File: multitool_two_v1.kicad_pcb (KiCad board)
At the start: 2 copper layers, 144.8 x 119.4 mm, 69 parts, among them J1 Conn_02x08_Odd_Even, SW1 SW_Push, SW2 SW_Push, SW3 SW_Push, SW4 SW_Push, SW5 SW_Push, SW6 SW_Push, SW7 SW_Push, SW8 SW_Push, U1 4017, U2 74LS74, U3 74LS74, U4 74LS74, U5 74LS74, U6 74HCT00, U7 74HCT00, U8 74HCT00

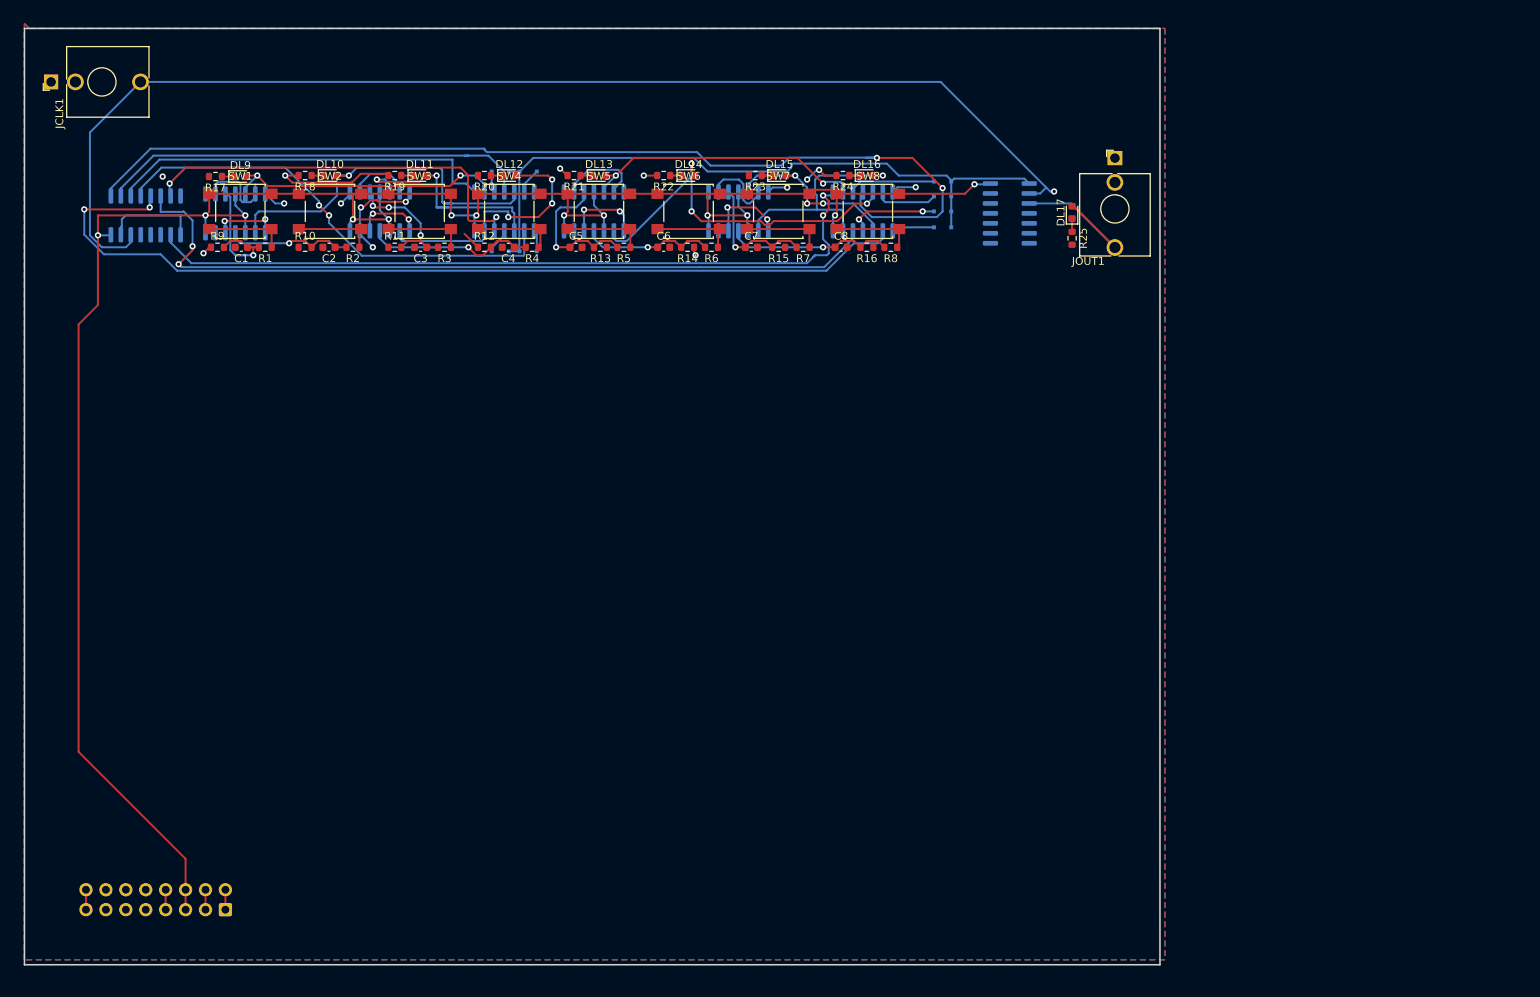
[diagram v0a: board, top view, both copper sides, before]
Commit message: committing with a bug
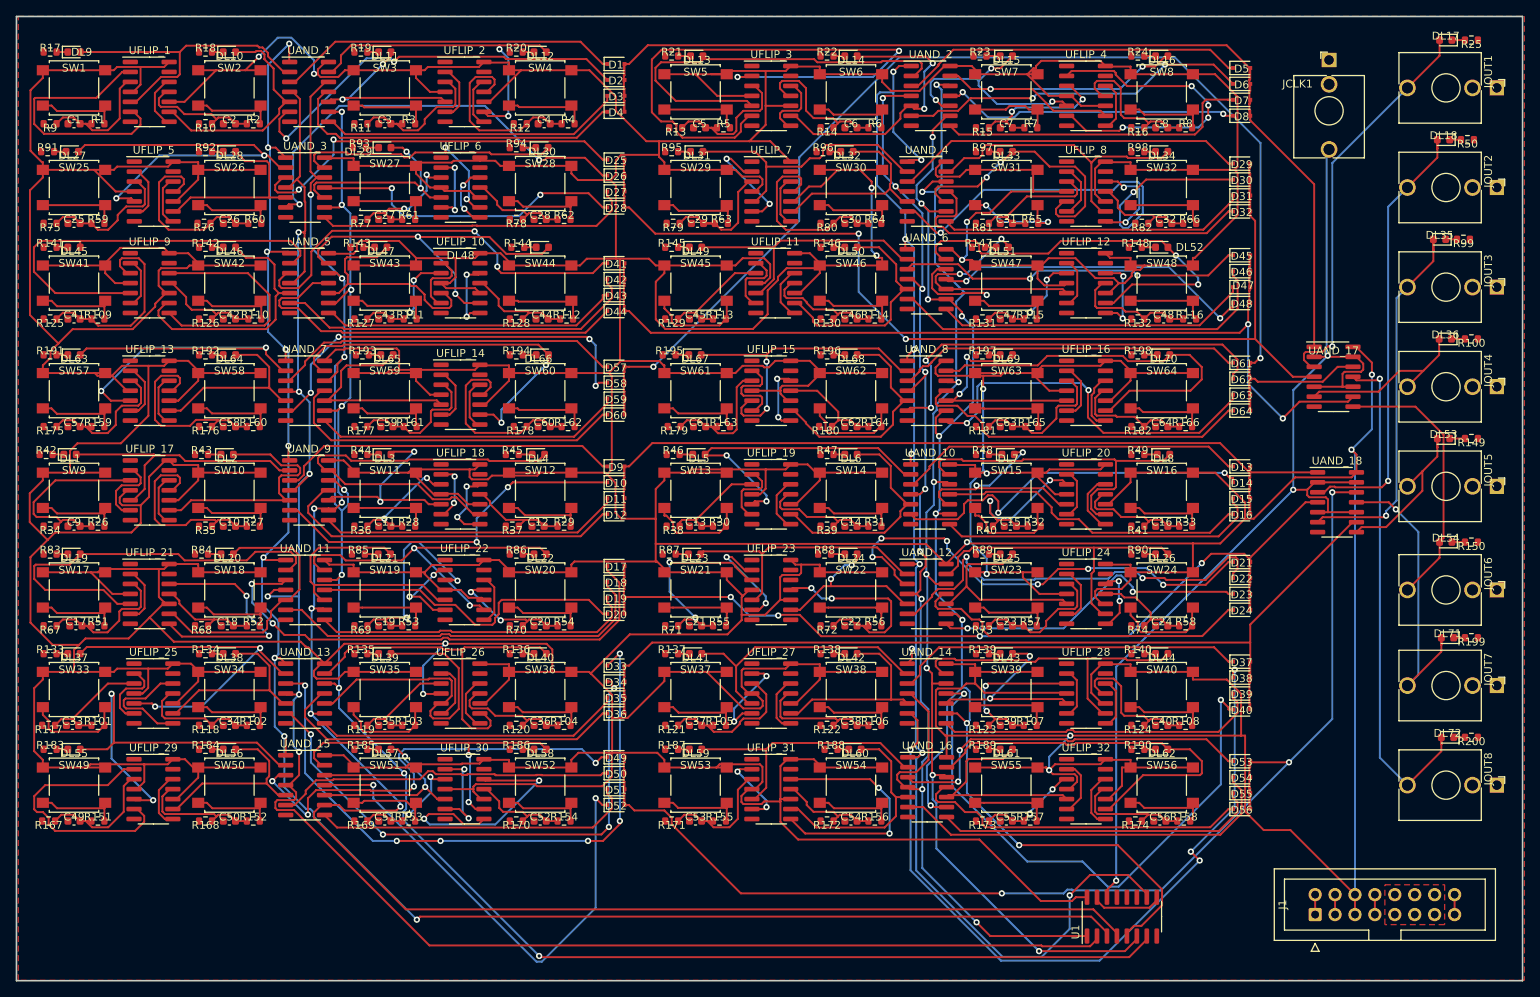
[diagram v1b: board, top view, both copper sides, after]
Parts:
- removed U2, U3, U4, U5: 74LS74, Package_SO:SOIC-14_3.9x8.7mm_P1.27mm
- removed U6, U7, U8: 74HCT00, Package_SO:SO-14_3.9x8.65mm_P1.27mm
- added C10: 1u, Capacitor_SMD:C_0603_1608Metric, F.Cu at (43.7, 83.3)
- added C11: 1u, Capacitor_SMD:C_0603_1608Metric, F.Cu at (63.5, 83.3)
- added C12: 1u, Capacitor_SMD:C_0603_1608Metric, F.Cu at (83.0, 83.3)
- added C13: 1u, Capacitor_SMD:C_0603_1608Metric, F.Cu at (103.1, 83.3)
- added C14: 1u, Capacitor_SMD:C_0603_1608Metric, F.Cu at (122.9, 83.3)
- added C15: 1u, Capacitor_SMD:C_0603_1608Metric, F.Cu at (143.3, 83.3)
- added C16: 1u, Capacitor_SMD:C_0603_1608Metric, F.Cu at (162.6, 83.3)
- added C17: 1u, Capacitor_SMD:C_0603_1608Metric, F.Cu at (24.1, 96.0)
- added C18: 1u, Capacitor_SMD:C_0603_1608Metric, F.Cu at (43.4, 96.0)
- added C19: 1u, Capacitor_SMD:C_0603_1608Metric, F.Cu at (63.5, 96.0)
- added C20: 1u, Capacitor_SMD:C_0603_1608Metric, F.Cu at (83.3, 96.0)
- added C21: 1u, Capacitor_SMD:C_0603_1608Metric, F.Cu at (103.1, 96.0)
- added C22: 1u, Capacitor_SMD:C_0603_1608Metric, F.Cu at (122.9, 96.0)
- added C23: 1u, Capacitor_SMD:C_0603_1608Metric, F.Cu at (142.7, 96.0)
- added C24: 1u, Capacitor_SMD:C_0603_1608Metric, F.Cu at (162.6, 96.0)
- added C25: 1u, Capacitor_SMD:C_0603_1608Metric, F.Cu at (23.9, 44.7)
- added C26: 1u, Capacitor_SMD:C_0603_1608Metric, F.Cu at (43.7, 44.7)
- added C27: 1u, Capacitor_SMD:C_0603_1608Metric, F.Cu at (63.5, 44.2)
- added C28: 1u, Capacitor_SMD:C_0603_1608Metric, F.Cu at (83.3, 44.2)
- added C29: 1u, Capacitor_SMD:C_0603_1608Metric, F.Cu at (103.4, 44.7)
- added C30: 1u, Capacitor_SMD:C_0603_1608Metric, F.Cu at (122.9, 44.7)
- added C31: 1u, Capacitor_SMD:C_0603_1608Metric, F.Cu at (142.7, 44.7)
- added C32: 1u, Capacitor_SMD:C_0603_1608Metric, F.Cu at (163.1, 44.7)
- added C33: 1u, Capacitor_SMD:C_0603_1608Metric, F.Cu at (23.7, 108.7)
- added C34: 1u, Capacitor_SMD:C_0603_1608Metric, F.Cu at (43.7, 108.7)
- added C35: 1u, Capacitor_SMD:C_0603_1608Metric, F.Cu at (63.5, 108.7)
- added C36: 1u, Capacitor_SMD:C_0603_1608Metric, F.Cu at (83.3, 108.7)
- added C37: 1u, Capacitor_SMD:C_0603_1608Metric, F.Cu at (103.1, 108.7)
- added C38: 1u, Capacitor_SMD:C_0603_1608Metric, F.Cu at (122.9, 108.7)
- added C39: 1u, Capacitor_SMD:C_0603_1608Metric, F.Cu at (142.7, 108.7)
- added C40: 1u, Capacitor_SMD:C_0603_1608Metric, F.Cu at (162.6, 108.7)
- added C41: 1u, Capacitor_SMD:C_0603_1608Metric, F.Cu at (23.9, 56.9)
- added C42: 1u, Capacitor_SMD:C_0603_1608Metric, F.Cu at (43.7, 56.9)
- added C43: 1u, Capacitor_SMD:C_0603_1608Metric, F.Cu at (63.5, 56.9)
- added C44: 1u, Capacitor_SMD:C_0603_1608Metric, F.Cu at (83.6, 56.9)
- added C45: 1u, Capacitor_SMD:C_0603_1608Metric, F.Cu at (103.1, 56.9)
- added C46: 1u, Capacitor_SMD:C_0603_1608Metric, F.Cu at (122.9, 56.9)
- added C47: 1u, Capacitor_SMD:C_0603_1608Metric, F.Cu at (142.7, 56.9)
- added C48: 1u, Capacitor_SMD:C_0603_1608Metric, F.Cu at (162.8, 56.9)
- added C49: 1u, Capacitor_SMD:C_0603_1608Metric, F.Cu at (23.9, 120.9)
- added C50: 1u, Capacitor_SMD:C_0603_1608Metric, F.Cu at (43.7, 120.9)
- added C51: 1u, Capacitor_SMD:C_0603_1608Metric, F.Cu at (63.5, 120.9)
- added C52: 1u, Capacitor_SMD:C_0603_1608Metric, F.Cu at (83.3, 120.9)
- added C53: 1u, Capacitor_SMD:C_0603_1608Metric, F.Cu at (103.1, 120.9)
- added C54: 1u, Capacitor_SMD:C_0603_1608Metric, F.Cu at (122.9, 120.9)
- added C55: 1u, Capacitor_SMD:C_0603_1608Metric, F.Cu at (142.7, 120.9)
- added C56: 1u, Capacitor_SMD:C_0603_1608Metric, F.Cu at (162.3, 120.9)
- added C57: 1u, Capacitor_SMD:C_0603_1608Metric, F.Cu at (23.9, 70.6)
- added C58: 1u, Capacitor_SMD:C_0603_1608Metric, F.Cu at (43.7, 70.6)
- added C59: 1u, Capacitor_SMD:C_0603_1608Metric, F.Cu at (63.8, 70.6)
- added C60: 1u, Capacitor_SMD:C_0603_1608Metric, F.Cu at (83.8, 70.6)
- added C61: 1u, Capacitor_SMD:C_0603_1608Metric, F.Cu at (103.6, 70.6)
- added C62: 1u, Capacitor_SMD:C_0603_1608Metric, F.Cu at (122.9, 70.6)
- added C63: 1u, Capacitor_SMD:C_0603_1608Metric, F.Cu at (142.7, 70.6)
- added C64: 1u, Capacitor_SMD:C_0603_1608Metric, F.Cu at (162.6, 70.6)
- added C9: 1u, Capacitor_SMD:C_0603_1608Metric, F.Cu at (23.9, 83.3)
- added D10: DIODE, Diode_SMD:D_SOD-323F, F.Cu at (93.0, 77.7)
- added D11: DIODE, Diode_SMD:D_SOD-323F, F.Cu at (93.0, 79.8)
- added D12: DIODE, Diode_SMD:D_SOD-323F, F.Cu at (93.0, 81.8)
- added D13: DIODE, Diode_SMD:D_SOD-323F, F.Cu at (172.7, 75.7)
- added D14: DIODE, Diode_SMD:D_SOD-323F, F.Cu at (172.7, 77.7)
- added D15: DIODE, Diode_SMD:D_SOD-323F, F.Cu at (172.7, 79.8)
- added D16: DIODE, Diode_SMD:D_SOD-323F, F.Cu at (172.7, 81.8)
- added D17: DIODE, Diode_SMD:D_SOD-323F, F.Cu at (93.0, 88.4)
- added D18: DIODE, Diode_SMD:D_SOD-323F, F.Cu at (93.0, 90.4)
- added D19: DIODE, Diode_SMD:D_SOD-323F, F.Cu at (93.0, 92.5)
- added D20: DIODE, Diode_SMD:D_SOD-323F, F.Cu at (93.0, 94.5)
- added D21: DIODE, Diode_SMD:D_SOD-323F, F.Cu at (172.7, 87.9)
- added D22: DIODE, Diode_SMD:D_SOD-323F, F.Cu at (172.7, 89.9)
- added D23: DIODE, Diode_SMD:D_SOD-323F, F.Cu at (172.7, 91.9)
- added D24: DIODE, Diode_SMD:D_SOD-323F, F.Cu at (172.7, 94.0)
- added D25: DIODE, Diode_SMD:D_SOD-323F, F.Cu at (93.0, 36.6)
- added D26: DIODE, Diode_SMD:D_SOD-323F, F.Cu at (93.0, 38.6)
- added D27: DIODE, Diode_SMD:D_SOD-323F, F.Cu at (93.0, 40.6)
- added D28: DIODE, Diode_SMD:D_SOD-323F, F.Cu at (93.0, 42.7)
- added D29: DIODE, Diode_SMD:D_SOD-323F, F.Cu at (172.7, 37.1)
- added D30: DIODE, Diode_SMD:D_SOD-323F, F.Cu at (172.7, 39.1)
- added D31: DIODE, Diode_SMD:D_SOD-323F, F.Cu at (172.7, 41.1)
- added D32: DIODE, Diode_SMD:D_SOD-323F, F.Cu at (172.7, 43.2)
- added D33: DIODE, Diode_SMD:D_SOD-323F, F.Cu at (93.0, 101.1)
- added D34: DIODE, Diode_SMD:D_SOD-323F, F.Cu at (93.0, 103.1)
- added D35: DIODE, Diode_SMD:D_SOD-323F, F.Cu at (93.0, 105.2)
- added D36: DIODE, Diode_SMD:D_SOD-323F, F.Cu at (93.0, 107.2)
- added D37: DIODE, Diode_SMD:D_SOD-323F, F.Cu at (172.7, 100.6)
- added D38: DIODE, Diode_SMD:D_SOD-323F, F.Cu at (172.7, 102.6)
- added D39: DIODE, Diode_SMD:D_SOD-323F, F.Cu at (172.7, 104.6)
- added D40: DIODE, Diode_SMD:D_SOD-323F, F.Cu at (172.7, 106.7)
- added D41: DIODE, Diode_SMD:D_SOD-323F, F.Cu at (93.0, 49.8)
- added D42: DIODE, Diode_SMD:D_SOD-323F, F.Cu at (93.0, 51.8)
- added D43: DIODE, Diode_SMD:D_SOD-323F, F.Cu at (93.0, 53.8)
- added D44: DIODE, Diode_SMD:D_SOD-323F, F.Cu at (93.0, 55.9)
- added D45: DIODE, Diode_SMD:D_SOD-323F, F.Cu at (172.7, 48.8)
- added D46: DIODE, Diode_SMD:D_SOD-323F, F.Cu at (172.7, 50.8)
- added D47: DIODE, Diode_SMD:D_SOD-323F, F.Cu at (172.7, 52.8)
- added D48: DIODE, Diode_SMD:D_SOD-323F, F.Cu at (172.7, 54.9)
- added D49: DIODE, Diode_SMD:D_SOD-323F, F.Cu at (93.0, 112.8)
- added D50: DIODE, Diode_SMD:D_SOD-323F, F.Cu at (93.0, 114.8)
- added D51: DIODE, Diode_SMD:D_SOD-323F, F.Cu at (93.0, 116.8)
- added D52: DIODE, Diode_SMD:D_SOD-323F, F.Cu at (93.0, 118.9)
- added D53: DIODE, Diode_SMD:D_SOD-323F, F.Cu at (172.7, 113.3)
- added D54: DIODE, Diode_SMD:D_SOD-323F, F.Cu at (172.7, 115.3)
- added D55: DIODE, Diode_SMD:D_SOD-323F, F.Cu at (172.7, 117.3)
- added D56: DIODE, Diode_SMD:D_SOD-323F, F.Cu at (172.7, 119.4)
- added D57: DIODE, Diode_SMD:D_SOD-323F, F.Cu at (93.0, 63.0)
- added D58: DIODE, Diode_SMD:D_SOD-323F, F.Cu at (93.0, 65.0)
- added D59: DIODE, Diode_SMD:D_SOD-323F, F.Cu at (93.0, 67.1)
- added D60: DIODE, Diode_SMD:D_SOD-323F, F.Cu at (93.0, 69.1)
- added D61: DIODE, Diode_SMD:D_SOD-323F, F.Cu at (172.7, 62.5)
- added D62: DIODE, Diode_SMD:D_SOD-323F, F.Cu at (172.7, 64.5)
- added D63: DIODE, Diode_SMD:D_SOD-323F, F.Cu at (172.7, 66.5)
- added D64: DIODE, Diode_SMD:D_SOD-323F, F.Cu at (172.7, 68.6)
- added D9: DIODE, Diode_SMD:D_SOD-323F, F.Cu at (93.0, 75.7)
- added DL1: LED, LED_SMD:LED_0603_1608Metric, F.Cu at (23.4, 74.2)
- added DL18: LED, LED_SMD:LED_0603_1608Metric, F.Cu at (198.5, 34.0)
- added DL19: LED, LED_SMD:LED_0603_1608Metric, F.Cu at (23.9, 86.9)
- added DL2: LED, LED_SMD:LED_0603_1608Metric, F.Cu at (43.4, 74.2)
- added DL20: LED, LED_SMD:LED_0603_1608Metric, F.Cu at (43.4, 86.9)
- added DL21: LED, LED_SMD:LED_0603_1608Metric, F.Cu at (63.4, 86.9)
- added DL22: LED, LED_SMD:LED_0603_1608Metric, F.Cu at (83.3, 86.9)
- added DL23: LED, LED_SMD:LED_0603_1608Metric, F.Cu at (103.0, 86.9)
- added DL24: LED, LED_SMD:LED_0603_1608Metric, F.Cu at (122.9, 86.9)
- added DL25: LED, LED_SMD:LED_0603_1608Metric, F.Cu at (142.7, 86.9)
- added DL26: LED, LED_SMD:LED_0603_1608Metric, F.Cu at (162.6, 86.9)
- added DL27: LED, LED_SMD:LED_0603_1608Metric, F.Cu at (23.6, 35.6)
- added DL28: LED, LED_SMD:LED_0603_1608Metric, F.Cu at (43.7, 35.6)
- added DL29: LED, LED_SMD:LED_0603_1608Metric, F.Cu at (63.5, 35.1)
- added DL3: LED, LED_SMD:LED_0603_1608Metric, F.Cu at (63.5, 74.2)
- added DL30: LED, LED_SMD:LED_0603_1608Metric, F.Cu at (83.5, 35.1)
- added DL31: LED, LED_SMD:LED_0603_1608Metric, F.Cu at (103.3, 35.6)
- added DL32: LED, LED_SMD:LED_0603_1608Metric, F.Cu at (122.4, 35.6)
- added DL33: LED, LED_SMD:LED_0603_1608Metric, F.Cu at (142.7, 35.6)
- added DL34: LED, LED_SMD:LED_0603_1608Metric, F.Cu at (162.6, 35.6)
- added DL35: LED, LED_SMD:LED_0603_1608Metric, F.Cu at (198.0, 46.7)
- added DL36: LED, LED_SMD:LED_0603_1608Metric, F.Cu at (198.7, 59.4)
- added DL37: LED, LED_SMD:LED_0603_1608Metric, F.Cu at (23.9, 99.6)
- added DL38: LED, LED_SMD:LED_0603_1608Metric, F.Cu at (43.7, 99.6)
- added DL39: LED, LED_SMD:LED_0603_1608Metric, F.Cu at (63.5, 99.6)
- added DL4: LED, LED_SMD:LED_0603_1608Metric, F.Cu at (83.1, 74.2)
- added DL40: LED, LED_SMD:LED_0603_1608Metric, F.Cu at (83.3, 99.6)
- added DL41: LED, LED_SMD:LED_0603_1608Metric, F.Cu at (103.1, 99.6)
- added DL42: LED, LED_SMD:LED_0603_1608Metric, F.Cu at (122.9, 99.6)
- added DL43: LED, LED_SMD:LED_0603_1608Metric, F.Cu at (142.7, 99.6)
- added DL44: LED, LED_SMD:LED_0603_1608Metric, F.Cu at (162.6, 99.6)
- added DL45: LED, LED_SMD:LED_0603_1608Metric, F.Cu at (23.9, 47.8)
- added DL46: LED, LED_SMD:LED_0603_1608Metric, F.Cu at (43.7, 47.8)
- added DL47: LED, LED_SMD:LED_0603_1608Metric, F.Cu at (63.0, 47.8)
- added DL48: LED, LED_SMD:LED_0603_1608Metric, F.Cu at (83.6, 47.8)
- added DL49: LED, LED_SMD:LED_0603_1608Metric, F.Cu at (103.1, 47.8)
- added DL5: LED, LED_SMD:LED_0603_1608Metric, F.Cu at (103.6, 74.2)
- added DL50: LED, LED_SMD:LED_0603_1608Metric, F.Cu at (122.9, 47.8)
- added DL51: LED, LED_SMD:LED_0603_1608Metric, F.Cu at (142.2, 47.8)
- added DL52: LED, LED_SMD:LED_0603_1608Metric, F.Cu at (162.6, 47.8)
- added DL53: LED, LED_SMD:LED_0603_1608Metric, F.Cu at (198.5, 72.1)
- added DL54: LED, LED_SMD:LED_0603_1608Metric, F.Cu at (198.8, 85.3)
- added DL55: LED, LED_SMD:LED_0603_1608Metric, F.Cu at (23.9, 111.8)
- added DL56: LED, LED_SMD:LED_0603_1608Metric, F.Cu at (43.7, 111.8)
- added DL57: LED, LED_SMD:LED_0603_1608Metric, F.Cu at (63.5, 111.8)
- added DL58: LED, LED_SMD:LED_0603_1608Metric, F.Cu at (83.3, 111.8)
- added DL59: LED, LED_SMD:LED_0603_1608Metric, F.Cu at (103.1, 111.8)
- added DL6: LED, LED_SMD:LED_0603_1608Metric, F.Cu at (122.9, 74.2)
- added DL60: LED, LED_SMD:LED_0603_1608Metric, F.Cu at (123.4, 111.8)
- added DL61: LED, LED_SMD:LED_0603_1608Metric, F.Cu at (142.7, 111.8)
- added DL62: LED, LED_SMD:LED_0603_1608Metric, F.Cu at (162.6, 111.8)
- added DL63: LED, LED_SMD:LED_0603_1608Metric, F.Cu at (23.9, 61.5)
- added DL64: LED, LED_SMD:LED_0603_1608Metric, F.Cu at (43.7, 61.5)
- added DL65: LED, LED_SMD:LED_0603_1608Metric, F.Cu at (63.8, 61.5)
- added DL66: LED, LED_SMD:LED_0603_1608Metric, F.Cu at (83.6, 61.5)
- added DL67: LED, LED_SMD:LED_0603_1608Metric, F.Cu at (103.0, 61.5)
- added DL68: LED, LED_SMD:LED_0603_1608Metric, F.Cu at (122.9, 61.5)
- added DL69: LED, LED_SMD:LED_0603_1608Metric, F.Cu at (142.7, 61.5)
- added DL7: LED, LED_SMD:LED_0603_1608Metric, F.Cu at (143.0, 74.2)
- added DL70: LED, LED_SMD:LED_0603_1608Metric, F.Cu at (162.8, 61.5)
- added DL71: LED, LED_SMD:LED_0603_1608Metric, F.Cu at (199.0, 97.5)
- added DL72: LED, LED_SMD:LED_0603_1608Metric, F.Cu at (199.0, 110.2)
- added DL8: LED, LED_SMD:LED_0603_1608Metric, F.Cu at (162.8, 74.2)
- added JOUT2: AudioJack2_SwitchT, Connector_Audio:Jack_3.5mm_QingPu_WQP-PJ398SM_Vertical_CircularHoles, F.Cu at (205.3, 40.1)
- added JOUT3: AudioJack2_SwitchT, Connector_Audio:Jack_3.5mm_QingPu_WQP-PJ398SM_Vertical_CircularHoles, F.Cu at (205.3, 52.8)
- added JOUT4: AudioJack2_SwitchT, Connector_Audio:Jack_3.5mm_QingPu_WQP-PJ398SM_Vertical_CircularHoles, F.Cu at (205.3, 65.5)
- added JOUT5: AudioJack2_SwitchT, Connector_Audio:Jack_3.5mm_QingPu_WQP-PJ398SM_Vertical_CircularHoles, F.Cu at (205.3, 78.2)
- added JOUT6: AudioJack2_SwitchT, Connector_Audio:Jack_3.5mm_QingPu_WQP-PJ398SM_Vertical_CircularHoles, F.Cu at (205.3, 91.4)
- added JOUT7: AudioJack2_SwitchT, Connector_Audio:Jack_3.5mm_QingPu_WQP-PJ398SM_Vertical_CircularHoles, F.Cu at (205.3, 103.6)
- added JOUT8: AudioJack2_SwitchT, Connector_Audio:Jack_3.5mm_QingPu_WQP-PJ398SM_Vertical_CircularHoles, F.Cu at (205.3, 116.3)
- added R100: 1k, Resistor_SMD:R_0603_1608Metric, F.Cu at (202.0, 59.4)
- added R101: 1k, Resistor_SMD:R_0603_1608Metric, F.Cu at (26.9, 108.7)
- added R102: 1k, Resistor_SMD:R_0603_1608Metric, F.Cu at (46.7, 108.7)
- added R103: 1k, Resistor_SMD:R_0603_1608Metric, F.Cu at (66.5, 108.7)
- added R104: 1k, Resistor_SMD:R_0603_1608Metric, F.Cu at (86.4, 108.7)
- added R105: 1k, Resistor_SMD:R_0603_1608Metric, F.Cu at (106.2, 108.7)
- added R106: 1k, Resistor_SMD:R_0603_1608Metric, F.Cu at (126.0, 108.7)
- added R107: 1k, Resistor_SMD:R_0603_1608Metric, F.Cu at (145.8, 108.7)
- added R108: 1k, Resistor_SMD:R_0603_1608Metric, F.Cu at (165.6, 108.7)
- added R109: 1k, Resistor_SMD:R_0603_1608Metric, F.Cu at (26.9, 56.9)
- added R110: 1k, Resistor_SMD:R_0603_1608Metric, F.Cu at (46.9, 56.9)
- added R111: 1k, Resistor_SMD:R_0603_1608Metric, F.Cu at (66.7, 56.9)
- added R112: 1k, Resistor_SMD:R_0603_1608Metric, F.Cu at (86.7, 56.9)
- added R113: 1k, Resistor_SMD:R_0603_1608Metric, F.Cu at (106.2, 56.9)
- added R114: 1k, Resistor_SMD:R_0603_1608Metric, F.Cu at (126.0, 56.9)
- added R115: 1k, Resistor_SMD:R_0603_1608Metric, F.Cu at (145.8, 56.9)
- added R116: 1k, Resistor_SMD:R_0603_1608Metric, F.Cu at (166.1, 56.9)
- added R117: 10k, Resistor_SMD:R_0603_1608Metric, F.Cu at (20.6, 108.7)
- added R118: 10k, Resistor_SMD:R_0603_1608Metric, F.Cu at (40.6, 108.7)
- added R119: 10k, Resistor_SMD:R_0603_1608Metric, F.Cu at (60.5, 108.7)
- added R120: 10k, Resistor_SMD:R_0603_1608Metric, F.Cu at (80.3, 108.7)
- added R121: 10k, Resistor_SMD:R_0603_1608Metric, F.Cu at (100.1, 108.7)
- added R122: 10k, Resistor_SMD:R_0603_1608Metric, F.Cu at (119.9, 108.7)
- added R123: 10k, Resistor_SMD:R_0603_1608Metric, F.Cu at (139.7, 108.7)
- added R124: 10k, Resistor_SMD:R_0603_1608Metric, F.Cu at (159.5, 108.7)
- added R125: 10k, Resistor_SMD:R_0603_1608Metric, F.Cu at (20.8, 56.9)
- added R126: 10k, Resistor_SMD:R_0603_1608Metric, F.Cu at (40.6, 56.9)
- added R127: 10k, Resistor_SMD:R_0603_1608Metric, F.Cu at (60.5, 56.9)
- added R128: 10k, Resistor_SMD:R_0603_1608Metric, F.Cu at (80.3, 56.9)
- added R129: 10k, Resistor_SMD:R_0603_1608Metric, F.Cu at (100.1, 56.9)
- added R130: 10k, Resistor_SMD:R_0603_1608Metric, F.Cu at (119.9, 56.9)
- added R131: 10k, Resistor_SMD:R_0603_1608Metric, F.Cu at (139.7, 56.9)
- added R132: 10k, Resistor_SMD:R_0603_1608Metric, F.Cu at (159.5, 56.9)
- added R133: 1k, Resistor_SMD:R_0603_1608Metric, F.Cu at (20.8, 99.6)
- added R134: 1k, Resistor_SMD:R_0603_1608Metric, F.Cu at (40.6, 99.6)
- added R135: 1k, Resistor_SMD:R_0603_1608Metric, F.Cu at (60.5, 99.6)
- added R136: 1k, Resistor_SMD:R_0603_1608Metric, F.Cu at (80.3, 99.6)
- added R137: 1k, Resistor_SMD:R_0603_1608Metric, F.Cu at (100.1, 99.6)
- added R138: 1k, Resistor_SMD:R_0603_1608Metric, F.Cu at (119.9, 99.6)
- added R139: 1k, Resistor_SMD:R_0603_1608Metric, F.Cu at (139.7, 99.6)
- added R140: 1k, Resistor_SMD:R_0603_1608Metric, F.Cu at (159.5, 99.6)
- added R141: 1k, Resistor_SMD:R_0603_1608Metric, F.Cu at (20.8, 47.8)
- added R142: 1k, Resistor_SMD:R_0603_1608Metric, F.Cu at (40.6, 47.8)
- added R143: 1k, Resistor_SMD:R_0603_1608Metric, F.Cu at (59.9, 47.8)
- added R144: 1k, Resistor_SMD:R_0603_1608Metric, F.Cu at (80.5, 47.8)
- added R145: 1k, Resistor_SMD:R_0603_1608Metric, F.Cu at (100.1, 47.8)
- added R146: 1k, Resistor_SMD:R_0603_1608Metric, F.Cu at (119.9, 47.8)
- added R147: 1k, Resistor_SMD:R_0603_1608Metric, F.Cu at (139.2, 47.8)
- added R148: 1k, Resistor_SMD:R_0603_1608Metric, F.Cu at (159.2, 47.8)
- added R149: 1k, Resistor_SMD:R_0603_1608Metric, F.Cu at (202.0, 72.1)
- added R150: 1k, Resistor_SMD:R_0603_1608Metric, F.Cu at (202.0, 85.3)
- added R151: 1k, Resistor_SMD:R_0603_1608Metric, F.Cu at (26.9, 120.9)
- added R152: 1k, Resistor_SMD:R_0603_1608Metric, F.Cu at (46.7, 120.9)
- added R153: 1k, Resistor_SMD:R_0603_1608Metric, F.Cu at (66.5, 120.9)
- added R154: 1k, Resistor_SMD:R_0603_1608Metric, F.Cu at (86.4, 120.9)
- added R155: 1k, Resistor_SMD:R_0603_1608Metric, F.Cu at (106.2, 120.9)
- added R156: 1k, Resistor_SMD:R_0603_1608Metric, F.Cu at (126.0, 120.9)
- added R157: 1k, Resistor_SMD:R_0603_1608Metric, F.Cu at (145.8, 120.9)
- added R158: 1k, Resistor_SMD:R_0603_1608Metric, F.Cu at (165.4, 120.9)
- added R159: 1k, Resistor_SMD:R_0603_1608Metric, F.Cu at (26.9, 70.6)
- added R160: 1k, Resistor_SMD:R_0603_1608Metric, F.Cu at (46.7, 70.6)
- added R161: 1k, Resistor_SMD:R_0603_1608Metric, F.Cu at (66.7, 70.6)
- added R162: 1k, Resistor_SMD:R_0603_1608Metric, F.Cu at (86.9, 70.6)
- added R163: 1k, Resistor_SMD:R_0603_1608Metric, F.Cu at (106.7, 70.6)
- added R164: 1k, Resistor_SMD:R_0603_1608Metric, F.Cu at (126.0, 70.6)
- added R165: 1k, Resistor_SMD:R_0603_1608Metric, F.Cu at (146.0, 70.6)
- added R166: 1k, Resistor_SMD:R_0603_1608Metric, F.Cu at (165.6, 70.6)
- added R167: 10k, Resistor_SMD:R_0603_1608Metric, F.Cu at (20.6, 120.9)
- added R168: 10k, Resistor_SMD:R_0603_1608Metric, F.Cu at (40.6, 120.9)
- added R169: 10k, Resistor_SMD:R_0603_1608Metric, F.Cu at (60.5, 120.9)
- added R170: 10k, Resistor_SMD:R_0603_1608Metric, F.Cu at (80.3, 120.9)
- added R171: 10k, Resistor_SMD:R_0603_1608Metric, F.Cu at (100.1, 120.9)
- added R172: 10k, Resistor_SMD:R_0603_1608Metric, F.Cu at (119.9, 120.9)
- added R173: 10k, Resistor_SMD:R_0603_1608Metric, F.Cu at (139.7, 120.9)
- added R174: 10k, Resistor_SMD:R_0603_1608Metric, F.Cu at (159.2, 120.9)
- added R175: 10k, Resistor_SMD:R_0603_1608Metric, F.Cu at (20.8, 70.6)
- added R176: 10k, Resistor_SMD:R_0603_1608Metric, F.Cu at (40.6, 70.6)
- added R177: 10k, Resistor_SMD:R_0603_1608Metric, F.Cu at (60.5, 70.6)
- added R178: 10k, Resistor_SMD:R_0603_1608Metric, F.Cu at (80.8, 70.6)
- added R179: 10k, Resistor_SMD:R_0603_1608Metric, F.Cu at (100.4, 70.6)
- added R180: 10k, Resistor_SMD:R_0603_1608Metric, F.Cu at (119.7, 70.6)
- added R181: 10k, Resistor_SMD:R_0603_1608Metric, F.Cu at (139.7, 70.6)
- added R182: 10k, Resistor_SMD:R_0603_1608Metric, F.Cu at (159.5, 70.6)
- added R183: 1k, Resistor_SMD:R_0603_1608Metric, F.Cu at (20.8, 111.8)
- added R184: 1k, Resistor_SMD:R_0603_1608Metric, F.Cu at (40.6, 111.8)
- added R185: 1k, Resistor_SMD:R_0603_1608Metric, F.Cu at (60.5, 111.8)
- added R186: 1k, Resistor_SMD:R_0603_1608Metric, F.Cu at (80.3, 111.8)
- added R187: 1k, Resistor_SMD:R_0603_1608Metric, F.Cu at (100.1, 111.8)
- added R188: 1k, Resistor_SMD:R_0603_1608Metric, F.Cu at (120.4, 111.8)
- added R189: 1k, Resistor_SMD:R_0603_1608Metric, F.Cu at (139.7, 111.8)
- added R190: 1k, Resistor_SMD:R_0603_1608Metric, F.Cu at (159.5, 111.8)
- added R191: 1k, Resistor_SMD:R_0603_1608Metric, F.Cu at (20.8, 61.5)
- added R192: 1k, Resistor_SMD:R_0603_1608Metric, F.Cu at (40.6, 61.5)
- added R193: 1k, Resistor_SMD:R_0603_1608Metric, F.Cu at (60.6, 61.5)
- added R194: 1k, Resistor_SMD:R_0603_1608Metric, F.Cu at (80.3, 61.5)
- added R195: 1k, Resistor_SMD:R_0603_1608Metric, F.Cu at (99.8, 61.5)
- added R196: 1k, Resistor_SMD:R_0603_1608Metric, F.Cu at (119.9, 61.5)
- added R197: 1k, Resistor_SMD:R_0603_1608Metric, F.Cu at (139.7, 61.5)
- added R198: 1k, Resistor_SMD:R_0603_1608Metric, F.Cu at (159.5, 61.5)
- added R199: 1k, Resistor_SMD:R_0603_1608Metric, F.Cu at (202.0, 97.5)
- added R200: 1k, Resistor_SMD:R_0603_1608Metric, F.Cu at (202.0, 110.2)
- added R26: 1k, Resistor_SMD:R_0603_1608Metric, F.Cu at (26.9, 83.3)
- added R27: 1k, Resistor_SMD:R_0603_1608Metric, F.Cu at (46.7, 83.3)
- added R28: 1k, Resistor_SMD:R_0603_1608Metric, F.Cu at (66.5, 83.3)
- added R29: 1k, Resistor_SMD:R_0603_1608Metric, F.Cu at (86.4, 83.3)
- added R30: 1k, Resistor_SMD:R_0603_1608Metric, F.Cu at (106.2, 83.3)
- added R31: 1k, Resistor_SMD:R_0603_1608Metric, F.Cu at (126.0, 83.3)
- added R32: 1k, Resistor_SMD:R_0603_1608Metric, F.Cu at (146.3, 83.3)
- added R33: 1k, Resistor_SMD:R_0603_1608Metric, F.Cu at (165.6, 83.3)
- added R34: 10k, Resistor_SMD:R_0603_1608Metric, F.Cu at (20.8, 83.3)
- added R35: 10k, Resistor_SMD:R_0603_1608Metric, F.Cu at (40.6, 83.3)
- added R36: 10k, Resistor_SMD:R_0603_1608Metric, F.Cu at (60.5, 83.3)
- added R37: 10k, Resistor_SMD:R_0603_1608Metric, F.Cu at (79.8, 83.3)
- added R38: 10k, Resistor_SMD:R_0603_1608Metric, F.Cu at (100.3, 83.3)
- added R39: 10k, Resistor_SMD:R_0603_1608Metric, F.Cu at (119.9, 83.3)
- added R40: 10k, Resistor_SMD:R_0603_1608Metric, F.Cu at (140.2, 83.3)
- added R41: 10k, Resistor_SMD:R_0603_1608Metric, F.Cu at (159.5, 83.3)
- added R42: 1k, Resistor_SMD:R_0603_1608Metric, F.Cu at (20.3, 74.2)
- added R43: 1k, Resistor_SMD:R_0603_1608Metric, F.Cu at (40.1, 74.2)
- added R44: 1k, Resistor_SMD:R_0603_1608Metric, F.Cu at (60.5, 74.2)
- added R45: 1k, Resistor_SMD:R_0603_1608Metric, F.Cu at (79.8, 74.2)
- added R46: 1k, Resistor_SMD:R_0603_1608Metric, F.Cu at (100.3, 74.2)
- added R47: 1k, Resistor_SMD:R_0603_1608Metric, F.Cu at (119.9, 74.2)
- added R48: 1k, Resistor_SMD:R_0603_1608Metric, F.Cu at (139.7, 74.2)
- added R49: 1k, Resistor_SMD:R_0603_1608Metric, F.Cu at (159.5, 74.2)
- added R50: 1k, Resistor_SMD:R_0603_1608Metric, F.Cu at (201.5, 34.0)
- added R51: 1k, Resistor_SMD:R_0603_1608Metric, F.Cu at (26.9, 96.0)
- added R52: 1k, Resistor_SMD:R_0603_1608Metric, F.Cu at (46.7, 96.0)
- added R53: 1k, Resistor_SMD:R_0603_1608Metric, F.Cu at (66.5, 96.0)
- added R54: 1k, Resistor_SMD:R_0603_1608Metric, F.Cu at (86.4, 96.0)
- added R55: 1k, Resistor_SMD:R_0603_1608Metric, F.Cu at (106.2, 96.0)
- added R56: 1k, Resistor_SMD:R_0603_1608Metric, F.Cu at (126.0, 96.0)
- added R57: 1k, Resistor_SMD:R_0603_1608Metric, F.Cu at (145.8, 96.0)
- added R58: 1k, Resistor_SMD:R_0603_1608Metric, F.Cu at (165.6, 96.0)
- added R59: 1k, Resistor_SMD:R_0603_1608Metric, F.Cu at (26.9, 44.7)
- added R60: 1k, Resistor_SMD:R_0603_1608Metric, F.Cu at (46.9, 44.7)
- added R61: 1k, Resistor_SMD:R_0603_1608Metric, F.Cu at (66.5, 44.2)
- added R62: 1k, Resistor_SMD:R_0603_1608Metric, F.Cu at (86.4, 44.2)
- added R63: 1k, Resistor_SMD:R_0603_1608Metric, F.Cu at (106.4, 44.7)
- added R64: 1k, Resistor_SMD:R_0603_1608Metric, F.Cu at (126.0, 44.7)
- added R65: 1k, Resistor_SMD:R_0603_1608Metric, F.Cu at (146.0, 44.7)
- added R66: 1k, Resistor_SMD:R_0603_1608Metric, F.Cu at (166.1, 44.7)
- added R67: 10k, Resistor_SMD:R_0603_1608Metric, F.Cu at (20.8, 96.0)
- added R68: 10k, Resistor_SMD:R_0603_1608Metric, F.Cu at (40.1, 96.0)
- added R69: 10k, Resistor_SMD:R_0603_1608Metric, F.Cu at (60.5, 96.0)
- added R70: 10k, Resistor_SMD:R_0603_1608Metric, F.Cu at (80.3, 96.0)
- added R71: 10k, Resistor_SMD:R_0603_1608Metric, F.Cu at (100.1, 96.0)
- added R72: 10k, Resistor_SMD:R_0603_1608Metric, F.Cu at (119.9, 96.0)
- added R73: 10k, Resistor_SMD:R_0603_1608Metric, F.Cu at (139.7, 96.0)
- added R74: 10k, Resistor_SMD:R_0603_1608Metric, F.Cu at (159.5, 96.0)
- added R75: 10k, Resistor_SMD:R_0603_1608Metric, F.Cu at (20.8, 44.7)
- added R76: 10k, Resistor_SMD:R_0603_1608Metric, F.Cu at (40.4, 44.7)
- added R77: 10k, Resistor_SMD:R_0603_1608Metric, F.Cu at (60.5, 44.2)
- added R78: 10k, Resistor_SMD:R_0603_1608Metric, F.Cu at (80.3, 44.2)
- added R79: 10k, Resistor_SMD:R_0603_1608Metric, F.Cu at (100.3, 44.7)
- added R80: 10k, Resistor_SMD:R_0603_1608Metric, F.Cu at (119.9, 44.7)
- added R81: 10k, Resistor_SMD:R_0603_1608Metric, F.Cu at (139.7, 44.7)
- added R82: 10k, Resistor_SMD:R_0603_1608Metric, F.Cu at (160.0, 44.7)
- added R83: 1k, Resistor_SMD:R_0603_1608Metric, F.Cu at (20.8, 86.9)
- added R84: 1k, Resistor_SMD:R_0603_1608Metric, F.Cu at (40.1, 86.9)
- added R85: 1k, Resistor_SMD:R_0603_1608Metric, F.Cu at (60.1, 86.9)
- added R86: 1k, Resistor_SMD:R_0603_1608Metric, F.Cu at (80.3, 86.9)
- added R87: 1k, Resistor_SMD:R_0603_1608Metric, F.Cu at (99.8, 86.9)
- added R88: 1k, Resistor_SMD:R_0603_1608Metric, F.Cu at (119.6, 86.9)
- added R89: 1k, Resistor_SMD:R_0603_1608Metric, F.Cu at (139.7, 86.9)
- added R90: 1k, Resistor_SMD:R_0603_1608Metric, F.Cu at (159.5, 86.9)
- added R91: 1k, Resistor_SMD:R_0603_1608Metric, F.Cu at (20.5, 35.6)
- added R92: 1k, Resistor_SMD:R_0603_1608Metric, F.Cu at (40.6, 35.6)
- added R93: 1k, Resistor_SMD:R_0603_1608Metric, F.Cu at (60.3, 35.1)
- added R94: 1k, Resistor_SMD:R_0603_1608Metric, F.Cu at (80.3, 35.1)
- added R95: 1k, Resistor_SMD:R_0603_1608Metric, F.Cu at (100.1, 35.6)
- added R96: 1k, Resistor_SMD:R_0603_1608Metric, F.Cu at (119.4, 35.6)
- added R97: 1k, Resistor_SMD:R_0603_1608Metric, F.Cu at (139.7, 35.6)
- added R98: 1k, Resistor_SMD:R_0603_1608Metric, F.Cu at (159.5, 35.6)
- added R99: 1k, Resistor_SMD:R_0603_1608Metric, F.Cu at (201.0, 46.7)
- added SW10: SW_Push, Button_Switch_SMD:SW_SPST_B3S-1000, F.Cu at (43.7, 78.7)
- added SW11: SW_Push, Button_Switch_SMD:SW_SPST_B3S-1000, F.Cu at (63.5, 78.7)
- added SW12: SW_Push, Button_Switch_SMD:SW_SPST_B3S-1000, F.Cu at (83.3, 78.7)
- added SW13: SW_Push, Button_Switch_SMD:SW_SPST_B3S-1000, F.Cu at (103.1, 78.7)
- added SW14: SW_Push, Button_Switch_SMD:SW_SPST_B3S-1000, F.Cu at (122.9, 78.7)
- added SW15: SW_Push, Button_Switch_SMD:SW_SPST_B3S-1000, F.Cu at (142.7, 78.7)
- added SW16: SW_Push, Button_Switch_SMD:SW_SPST_B3S-1000, F.Cu at (162.6, 78.7)
- added SW17: SW_Push, Button_Switch_SMD:SW_SPST_B3S-1000, F.Cu at (23.9, 91.4)
- added SW18: SW_Push, Button_Switch_SMD:SW_SPST_B3S-1000, F.Cu at (43.7, 91.4)
- added SW19: SW_Push, Button_Switch_SMD:SW_SPST_B3S-1000, F.Cu at (63.5, 91.4)
- added SW20: SW_Push, Button_Switch_SMD:SW_SPST_B3S-1000, F.Cu at (83.3, 91.4)
- added SW21: SW_Push, Button_Switch_SMD:SW_SPST_B3S-1000, F.Cu at (103.1, 91.4)
- added SW22: SW_Push, Button_Switch_SMD:SW_SPST_B3S-1000, F.Cu at (122.9, 91.4)
- added SW23: SW_Push, Button_Switch_SMD:SW_SPST_B3S-1000, F.Cu at (142.7, 91.4)
- added SW24: SW_Push, Button_Switch_SMD:SW_SPST_B3S-1000, F.Cu at (162.6, 91.4)
- added SW25: SW_Push, Button_Switch_SMD:SW_SPST_B3S-1000, F.Cu at (23.9, 40.1)
- added SW26: SW_Push, Button_Switch_SMD:SW_SPST_B3S-1000, F.Cu at (43.7, 40.1)
- added SW27: SW_Push, Button_Switch_SMD:SW_SPST_B3S-1000, F.Cu at (63.5, 39.6)
- added SW28: SW_Push, Button_Switch_SMD:SW_SPST_B3S-1000, F.Cu at (83.3, 39.6)
- added SW29: SW_Push, Button_Switch_SMD:SW_SPST_B3S-1000, F.Cu at (103.1, 40.1)
- added SW30: SW_Push, Button_Switch_SMD:SW_SPST_B3S-1000, F.Cu at (122.9, 40.1)
- added SW31: SW_Push, Button_Switch_SMD:SW_SPST_B3S-1000, F.Cu at (142.7, 40.1)
- added SW32: SW_Push, Button_Switch_SMD:SW_SPST_B3S-1000, F.Cu at (162.6, 40.1)
- added SW33: SW_Push, Button_Switch_SMD:SW_SPST_B3S-1000, F.Cu at (23.9, 104.1)
- added SW34: SW_Push, Button_Switch_SMD:SW_SPST_B3S-1000, F.Cu at (43.7, 104.1)
- added SW35: SW_Push, Button_Switch_SMD:SW_SPST_B3S-1000, F.Cu at (63.5, 104.1)
- added SW36: SW_Push, Button_Switch_SMD:SW_SPST_B3S-1000, F.Cu at (83.3, 104.1)
- added SW37: SW_Push, Button_Switch_SMD:SW_SPST_B3S-1000, F.Cu at (103.1, 104.1)
- added SW38: SW_Push, Button_Switch_SMD:SW_SPST_B3S-1000, F.Cu at (122.9, 104.1)
- added SW39: SW_Push, Button_Switch_SMD:SW_SPST_B3S-1000, F.Cu at (142.7, 104.1)
- added SW40: SW_Push, Button_Switch_SMD:SW_SPST_B3S-1000, F.Cu at (162.6, 104.1)
- added SW41: SW_Push, Button_Switch_SMD:SW_SPST_B3S-1000, F.Cu at (23.9, 52.3)
- added SW42: SW_Push, Button_Switch_SMD:SW_SPST_B3S-1000, F.Cu at (43.7, 52.3)
- added SW43: SW_Push, Button_Switch_SMD:SW_SPST_B3S-1000, F.Cu at (63.5, 52.3)
- added SW44: SW_Push, Button_Switch_SMD:SW_SPST_B3S-1000, F.Cu at (83.3, 52.3)
- added SW45: SW_Push, Button_Switch_SMD:SW_SPST_B3S-1000, F.Cu at (103.1, 52.3)
- added SW46: SW_Push, Button_Switch_SMD:SW_SPST_B3S-1000, F.Cu at (122.9, 52.3)
- added SW47: SW_Push, Button_Switch_SMD:SW_SPST_B3S-1000, F.Cu at (142.7, 52.3)
- added SW48: SW_Push, Button_Switch_SMD:SW_SPST_B3S-1000, F.Cu at (162.6, 52.3)
- added SW49: SW_Push, Button_Switch_SMD:SW_SPST_B3S-1000, F.Cu at (23.9, 116.3)
- added SW50: SW_Push, Button_Switch_SMD:SW_SPST_B3S-1000, F.Cu at (43.7, 116.3)
- added SW51: SW_Push, Button_Switch_SMD:SW_SPST_B3S-1000, F.Cu at (63.5, 116.3)
- added SW52: SW_Push, Button_Switch_SMD:SW_SPST_B3S-1000, F.Cu at (83.3, 116.3)
- added SW53: SW_Push, Button_Switch_SMD:SW_SPST_B3S-1000, F.Cu at (103.1, 116.3)
- added SW54: SW_Push, Button_Switch_SMD:SW_SPST_B3S-1000, F.Cu at (122.9, 116.3)
- added SW55: SW_Push, Button_Switch_SMD:SW_SPST_B3S-1000, F.Cu at (142.7, 116.3)
- added SW56: SW_Push, Button_Switch_SMD:SW_SPST_B3S-1000, F.Cu at (162.6, 116.3)
- added SW57: SW_Push, Button_Switch_SMD:SW_SPST_B3S-1000, F.Cu at (23.9, 66.0)
- added SW58: SW_Push, Button_Switch_SMD:SW_SPST_B3S-1000, F.Cu at (43.7, 66.0)
- added SW59: SW_Push, Button_Switch_SMD:SW_SPST_B3S-1000, F.Cu at (63.5, 66.0)
- added SW60: SW_Push, Button_Switch_SMD:SW_SPST_B3S-1000, F.Cu at (83.3, 66.0)
- added SW61: SW_Push, Button_Switch_SMD:SW_SPST_B3S-1000, F.Cu at (103.1, 66.0)
- added SW62: SW_Push, Button_Switch_SMD:SW_SPST_B3S-1000, F.Cu at (122.9, 66.0)
- added SW63: SW_Push, Button_Switch_SMD:SW_SPST_B3S-1000, F.Cu at (142.7, 66.0)
- added SW64: SW_Push, Button_Switch_SMD:SW_SPST_B3S-1000, F.Cu at (162.6, 66.0)
- added SW9: SW_Push, Button_Switch_SMD:SW_SPST_B3S-1000, F.Cu at (23.9, 78.7)
- added UAND_1: 74HCT00, Package_SO:SO-14_3.9x8.65mm_P1.27mm, F.Cu at (53.8, 27.9)
- added UAND_10: 74HCT00, Package_SO:SO-14_3.9x8.65mm_P1.27mm, F.Cu at (133.0, 79.2)
- added UAND_11: 74HCT00, Package_SO:SO-14_3.9x8.65mm_P1.27mm, F.Cu at (53.3, 91.4)
- added UAND_12: 74HCT00, Package_SO:SO-14_3.9x8.65mm_P1.27mm, F.Cu at (132.6, 91.9)
- added UAND_13: 74HCT00, Package_SO:SO-14_3.9x8.65mm_P1.27mm, F.Cu at (53.3, 104.6)
- added UAND_14: 74HCT00, Package_SO:SO-14_3.9x8.65mm_P1.27mm, F.Cu at (132.6, 104.6)
- added UAND_15: 74HCT00, Package_SO:SO-14_3.9x8.65mm_P1.27mm, F.Cu at (53.3, 116.3)
- added UAND_16: 74HCT00, Package_SO:SO-14_3.9x8.65mm_P1.27mm, F.Cu at (132.7, 116.6)
- added UAND_17: 74HCT00, Package_SO:SO-14_3.9x8.65mm_P1.27mm, F.Cu at (184.5, 64.3)
- added UAND_18: 74HCT00, Package_SO:SO-14_3.9x8.65mm_P1.27mm, F.Cu at (184.9, 80.3)
- added UAND_2: 74HCT00, Package_SO:SO-14_3.9x8.65mm_P1.27mm, F.Cu at (133.1, 28.4)
- added UAND_3: 74HCT00, Package_SO:SO-14_3.9x8.65mm_P1.27mm, F.Cu at (53.3, 40.1)
- added UAND_4: 74HCT00, Package_SO:SO-14_3.9x8.65mm_P1.27mm, F.Cu at (132.6, 40.6)
- added UAND_5: 74HCT00, Package_SO:SO-14_3.9x8.65mm_P1.27mm, F.Cu at (53.8, 52.3)
- added UAND_6: 74HCT00, Package_SO:SO-14_3.9x8.65mm_P1.27mm, F.Cu at (132.6, 51.8)
- added UAND_7: 74HCT00, Package_SO:SO-14_3.9x8.65mm_P1.27mm, F.Cu at (53.3, 66.0)
- added UAND_8: 74HCT00, Package_SO:SO-14_3.9x8.65mm_P1.27mm, F.Cu at (132.6, 66.0)
- added UAND_9: 74HCT00, Package_SO:SO-14_3.9x8.65mm_P1.27mm, F.Cu at (53.8, 78.7)
- added UFLIP_1: 74LS74, Package_SO:SOIC-14_3.9x8.7mm_P1.27mm, F.Cu at (33.5, 27.9)
- added UFLIP_10: 74LS74, Package_SO:SOIC-14_3.9x8.7mm_P1.27mm, F.Cu at (73.2, 52.3)
- added UFLIP_11: 74LS74, Package_SO:SOIC-14_3.9x8.7mm_P1.27mm, F.Cu at (113.3, 52.3)
- added UFLIP_12: 74LS74, Package_SO:SOIC-14_3.9x8.7mm_P1.27mm, F.Cu at (152.9, 52.3)
- added UFLIP_13: 74LS74, Package_SO:SOIC-14_3.9x8.7mm_P1.27mm, F.Cu at (33.5, 66.0)
- added UFLIP_14: 74LS74, Package_SO:SOIC-14_3.9x8.7mm_P1.27mm, F.Cu at (73.2, 66.5)
- added UFLIP_15: 74LS74, Package_SO:SOIC-14_3.9x8.7mm_P1.27mm, F.Cu at (112.8, 66.0)
- added UFLIP_16: 74LS74, Package_SO:SOIC-14_3.9x8.7mm_P1.27mm, F.Cu at (152.9, 66.0)
- added UFLIP_17: 74LS74, Package_SO:SOIC-14_3.9x8.7mm_P1.27mm, F.Cu at (33.5, 78.7)
- added UFLIP_18: 74LS74, Package_SO:SOIC-14_3.9x8.7mm_P1.27mm, F.Cu at (73.2, 79.2)
- added UFLIP_19: 74LS74, Package_SO:SOIC-14_3.9x8.7mm_P1.27mm, F.Cu at (112.8, 79.2)
- added UFLIP_2: 74LS74, Package_SO:SOIC-14_3.9x8.7mm_P1.27mm, F.Cu at (73.7, 27.9)
- added UFLIP_20: 74LS74, Package_SO:SOIC-14_3.9x8.7mm_P1.27mm, F.Cu at (152.9, 79.2)
- added UFLIP_21: 74LS74, Package_SO:SOIC-14_3.9x8.7mm_P1.27mm, F.Cu at (33.5, 91.9)
- added UFLIP_22: 74LS74, Package_SO:SOIC-14_3.9x8.7mm_P1.27mm, F.Cu at (73.7, 91.4)
- added UFLIP_23: 74LS74, Package_SO:SOIC-14_3.9x8.7mm_P1.27mm, F.Cu at (112.8, 91.4)
- added UFLIP_24: 74LS74, Package_SO:SOIC-14_3.9x8.7mm_P1.27mm, F.Cu at (152.9, 91.9)
- added UFLIP_25: 74LS74, Package_SO:SOIC-14_3.9x8.7mm_P1.27mm, F.Cu at (34.0, 104.6)
- added UFLIP_26: 74LS74, Package_SO:SOIC-14_3.9x8.7mm_P1.27mm, F.Cu at (73.2, 104.6)
- added UFLIP_27: 74LS74, Package_SO:SOIC-14_3.9x8.7mm_P1.27mm, F.Cu at (112.8, 104.6)
- added UFLIP_28: 74LS74, Package_SO:SOIC-14_3.9x8.7mm_P1.27mm, F.Cu at (152.9, 104.6)
- added UFLIP_29: 74LS74, Package_SO:SOIC-14_3.9x8.7mm_P1.27mm, F.Cu at (34.0, 116.8)
- added UFLIP_3: 74LS74, Package_SO:SOIC-14_3.9x8.7mm_P1.27mm, F.Cu at (112.8, 28.4)
- added UFLIP_30: 74LS74, Package_SO:SOIC-14_3.9x8.7mm_P1.27mm, F.Cu at (73.7, 116.8)
- added UFLIP_31: 74LS74, Package_SO:SOIC-14_3.9x8.7mm_P1.27mm, F.Cu at (112.8, 116.8)
- added UFLIP_32: 74LS74, Package_SO:SOIC-14_3.9x8.7mm_P1.27mm, F.Cu at (152.9, 116.8)
- added UFLIP_4: 74LS74, Package_SO:SOIC-14_3.9x8.7mm_P1.27mm, F.Cu at (152.9, 28.4)
- added UFLIP_5: 74LS74, Package_SO:SOIC-14_3.9x8.7mm_P1.27mm, F.Cu at (34.0, 40.6)
- added UFLIP_6: 74LS74, Package_SO:SOIC-14_3.9x8.7mm_P1.27mm, F.Cu at (73.2, 40.1)
- added UFLIP_7: 74LS74, Package_SO:SOIC-14_3.9x8.7mm_P1.27mm, F.Cu at (112.8, 40.6)
- added UFLIP_8: 74LS74, Package_SO:SOIC-14_3.9x8.7mm_P1.27mm, F.Cu at (152.9, 40.6)
- added UFLIP_9: 74LS74, Package_SO:SOIC-14_3.9x8.7mm_P1.27mm, F.Cu at (33.5, 52.3)
- D1, D2, D3, D4, D5, D6, D7, D8, J1, U1: moved to F.Cu
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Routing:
- net +5V: track 284.9 -> 2336.7 mm, vias 13 -> 16
- net count_1: track 49.8 -> 232.6 mm, vias 0 -> 9
- net count_4: track 52.3 -> 233.8 mm, vias 2 -> 8
- net count_2: track 55.6 -> 235.0 mm, vias 0 -> 6
- net count_3: track 59.6 -> 233.2 mm, vias 2 -> 9
- net Net-(D57-Pad2): track 0.00 -> 169.9 mm, vias 0 -> 2
- net Net-(D49-Pad2): track 0.00 -> 162.3 mm, vias 0 -> 3
- net Net-(D25-Pad2): track 0.00 -> 139.2 mm, vias 0 -> 2
- net Net-(D41-Pad2): track 0.00 -> 126.4 mm, vias 0 -> 2
- net Net-(D33-Pad2): track 0.00 -> 126.3 mm
- net Net-(D17-Pad2): track 0.00 -> 119.8 mm, vias 0 -> 4
- net Net-(D10-Pad2): track 0.00 -> 112.2 mm
- net Net-(D38-Pad1): track 0.00 -> 96.3 mm, vias 0 -> 4
- net Net-(D33-Pad1): track 0.00 -> 82.3 mm, vias 0 -> 6
- net Net-(UFLIP_3-Pad2): track 0.00 -> 79.0 mm, vias 0 -> 2
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- removed copper zone on B.Cu, net GND
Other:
- board size 144.8 x 119.4 mm -> 192 x 122.9 mm
